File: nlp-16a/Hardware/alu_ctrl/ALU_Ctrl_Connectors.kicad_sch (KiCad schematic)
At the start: 83 parts, among them J1 Screw_Terminal_01x02, J10 Conn_02x08_Odd_Even, J2 Conn_02x20_Odd_Even, J3 Conn_02x10_Counter_Clockwise, J4 Conn_02x10_Counter_Clockwise, J5 Conn_02x10_Counter_Clockwise, J6 Conn_02x10_Counter_Clockwise, J7 Conn_02x10_Counter_Clockwise, J8 Conn_02x08_Odd_Even, J9 Conn_02x08_Odd_Even, U28 CD74HC00

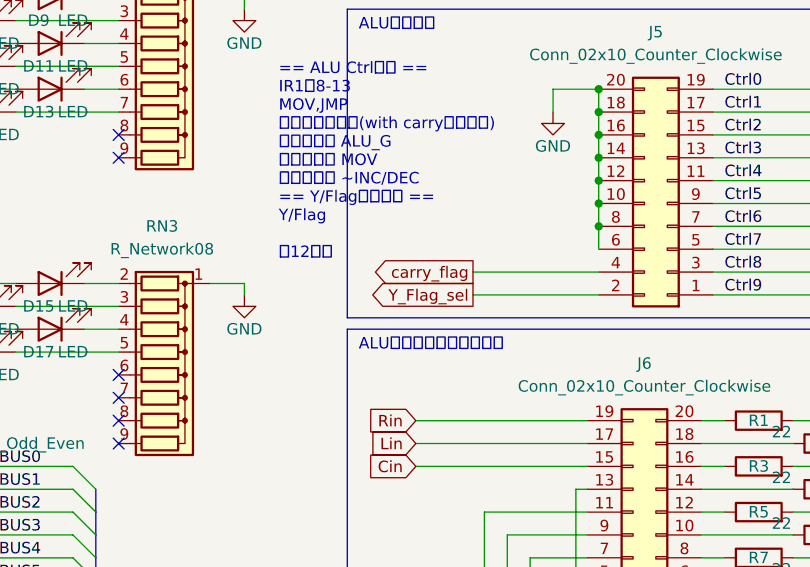
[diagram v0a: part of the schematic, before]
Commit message: 基板の途中経過
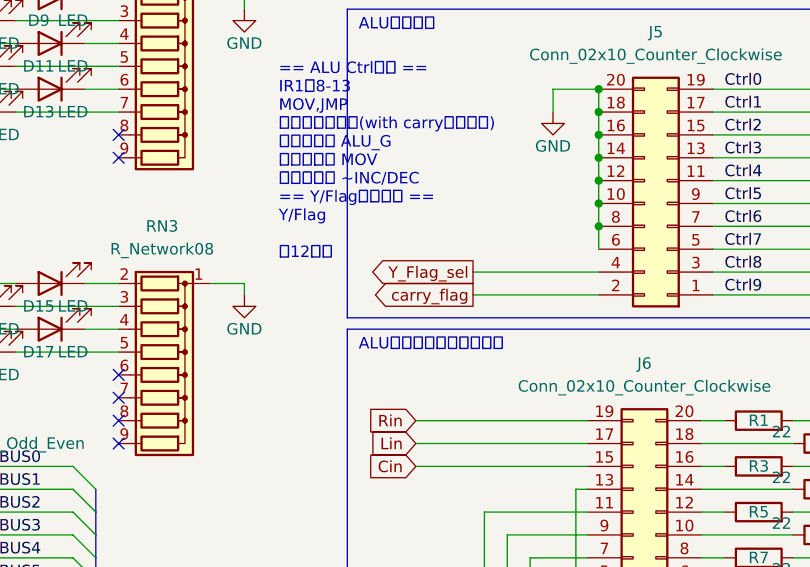
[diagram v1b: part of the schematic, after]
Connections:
- net Y_Flag_sel: now also J5.4 (Pin_4); no longer J5.2 (Pin_2)
- net carry_flag: now also J5.2 (Pin_2); no longer J5.4 (Pin_4)
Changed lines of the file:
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@@
     )
   )
-  (global_label "carry_flag" (shape output) (at 218.44 96.52 180) (fields_autoplaced)
+  (global_label "carry_flag" (shape output) (at 218.44 99.06 180) (fields_autoplaced)
     (effects (font (size 1.27 1.27)) (justify right))
-    (property "Intersheet References" "${INTERSHEET_REFS}" (id 0) (at 206.5926 96.4406 0)
+    (property "Intersheet References" "${INTERSHEET_REFS}" (id 0) (at 206.5926 98.9806 0)
       (effects (font (size 1.27 1.27)) (justify right) hide)
     )
@@
     )
   )
-  (global_label "Y_Flag_sel" (shape output) (at 218.44 99.06 180) (fields_autoplaced)
+  (global_label "Y_Flag_sel" (shape output) (at 218.44 96.52 180) (fields_autoplaced)
     (effects (font (size 1.27 1.27)) (justify right))
-    (property "Intersheet References" "${INTERSHEET_REFS}" (id 0) (at 206.1693 98.9806 0)
+    (property "Intersheet References" "${INTERSHEET_REFS}" (id 0) (at 206.1693 96.4406 0)
       (effects (font (size 1.27 1.27)) (justify right) hide)
     )
